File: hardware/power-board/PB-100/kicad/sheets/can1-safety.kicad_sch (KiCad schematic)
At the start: 2 parts

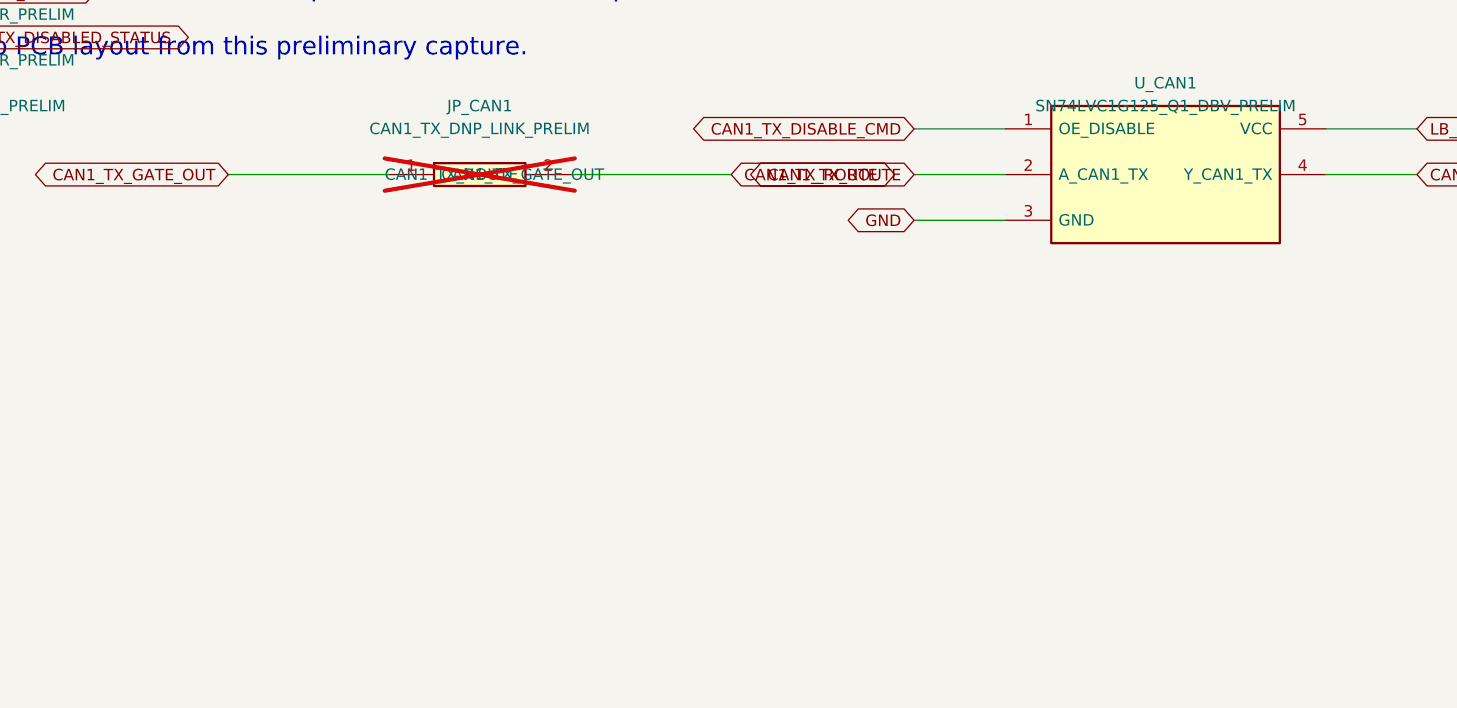
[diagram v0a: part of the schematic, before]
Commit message: fix
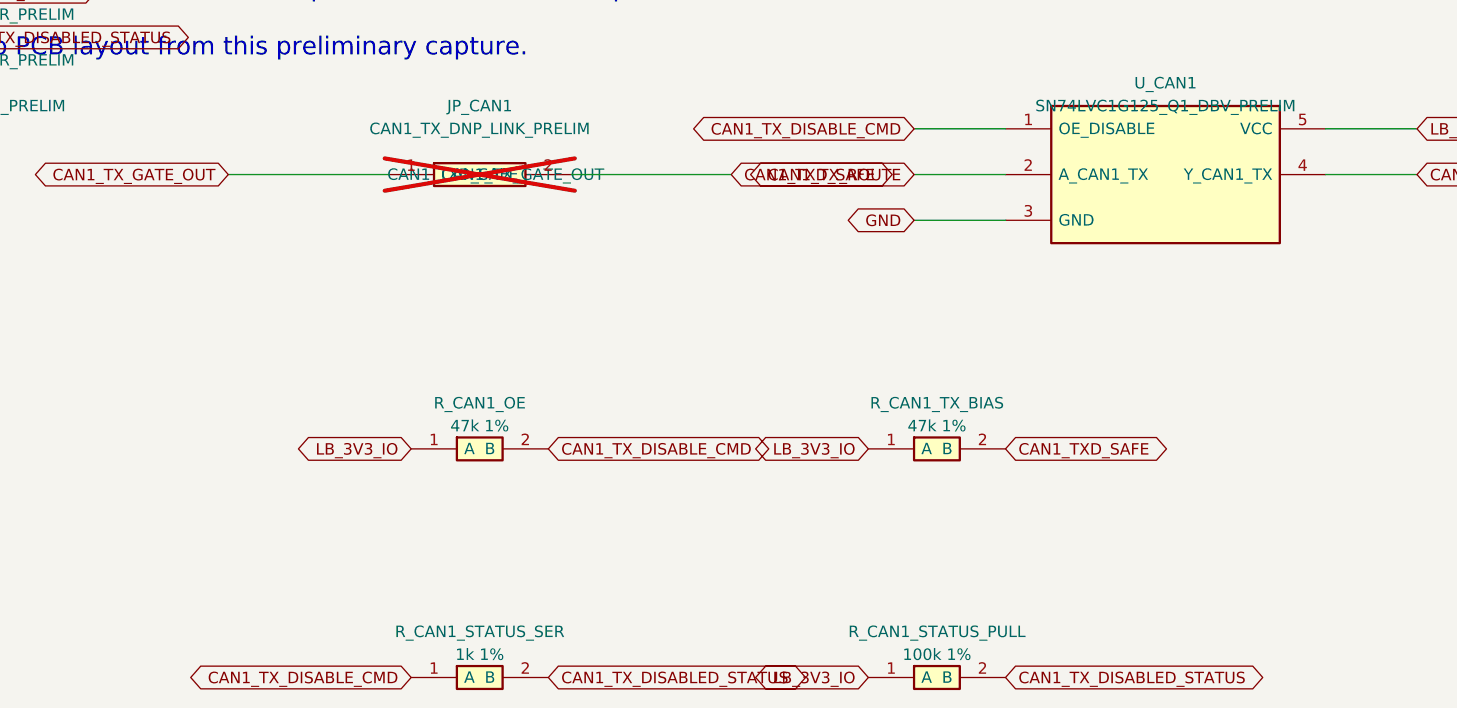
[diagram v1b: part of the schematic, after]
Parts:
- added R_CAN1_OE, R_CAN1_TX_BIAS: 47k 1%, PB100:R0402, symbol PB100:PB100_CAN1_SAFETY_RESISTOR_PRELIM
- added R_CAN1_STATUS_PULL: 100k 1%, PB100:R0402, symbol PB100:PB100_CAN1_SAFETY_RESISTOR_PRELIM
- added R_CAN1_STATUS_SER: 1k 1%, PB100:R0402, symbol PB100:PB100_CAN1_SAFETY_RESISTOR_PRELIM
- JP_CAN1: footprint (none) -> PB100:R0603_DNP_LINK_1608Metric
- U_CAN1: footprint (none) -> PB100:SOT-23-5_DBV_TI
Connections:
- net CAN1_TX_DISABLED_STATUS: now also R_CAN1_STATUS_PULL.2 (B), R_CAN1_STATUS_SER.2 (B)
- net CAN1_TX_DISABLE_CMD: now also R_CAN1_OE.2 (B), R_CAN1_STATUS_SER.1 (A)
- net CAN1_TX_ROUTE: no longer JP_CAN1.2 (CAN1_TX_ROUTE)
- net LB_3V3_IO: now also R_CAN1_OE.1 (A), R_CAN1_STATUS_PULL.1 (A), R_CAN1_TX_BIAS.1 (A)
- new net CAN1_TXD_SAFE: JP_CAN1.2 (CAN1_TXD_SAFE), R_CAN1_TX_BIAS.2 (B)
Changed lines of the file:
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@@
     (property "Reference" "JP_CAN1" (at 76.20 53.34 0) (effects (font (size 1.27 1.27))))
     (property "Value" "CAN1_TX_DNP_LINK_PRELIM" (at 76.20 55.88 0) (effects (font (size 1.27 1.27))))
-    (property "Footprint" "" (at 76.20 66.04 0) (effects (font (size 1.27 1.27)) hide))
+    (property "Footprint" "PB100:R0603_DNP_LINK_1608Metric" (at 76.20 66.04 0) (effects (font (size 1.27 1.27)) hide))
     (property "Datasheet" "../PB-100-can1-tx-disable.md" (at 76.20 68.58 0) (effects (font (size 1.27 1.27)) hide))
     (pin "1")
@@
   (global_label "CAN1_TX_GATE_OUT" (shape bidirectional) (at 48.26 60.96 0) (fields_autoplaced) (effects (font (size 1.27 1.27)) (justify right)) (property "Intersheetrefs" "${INTERSHEET_REFS}" (at 48.26 60.96 0) (effects (font (size 1.27 1.27)) hide)))
   (wire (pts (xy 86.36 60.96) (xy 104.14 60.96)) (stroke (width 0) (type default)))
-  (global_label "CAN1_TX_ROUTE" (shape bidirectional) (at 104.14 60.96 0) (fields_autoplaced) (effects (font (size 1.27 1.27)) (justify left)) (property "Intersheetrefs" "${INTERSHEET_REFS}" (at 104.14 60.96 0) (effects (font (size 1.27 1.27)) hide)))
+  (global_label "CAN1_TXD_SAFE" (shape bidirectional) (at 104.14 60.96 0) (fields_autoplaced) (effects (font (size 1.27 1.27)) (justify left)) (property "Intersheetrefs" "${INTERSHEET_REFS}" (at 104.14 60.96 0) (effects (font (size 1.27 1.27)) hide)))
   (symbol
     (lib_id "PB100:PB100_SN74LVC1G125_Q1_DBV_PRELIM")
@@
     (property "Reference" "U_CAN1" (at 152.40 50.80 0) (effects (font (size 1.27 1.27))))
     (property "Value" "SN74LVC1G125_Q1_DBV_PRELIM" (at 152.40 53.34 0) (effects (font (size 1.27 1.27))))
-    (property "Footprint" "" (at 152.40 71.12 0) (effects (font (size 1.27 1.27)) hide))
+    (property "Footprint" "PB100:SOT-23-5_DBV_TI" (at 152.40 71.12 0) (effects (font (size 1.27 1.27)) hide))
     (property "Datasheet" "https://www.ti.com/lit/ds/symlink/sn74lvc1g125-q1.pdf" (at 152.40 73.66 0) (effects (font (size 1.27 1.27)) hide))
     (pin "1")
@@
   (global_label "LB_3V3_IO" (shape bidirectional) (at 180.34 55.88 0) (fields_autoplaced) (effects (font (size 1.27 1.27)) (justify left)) (property "Intersheetrefs" "${INTERSHEET_REFS}" (at 180.34 55.88 0) (effects (font (size 1.27 1.27)) hide)))
   (symbol
+    (lib_id "PB100:PB100_CAN1_SAFETY_RESISTOR_PRELIM")
+    (at 76.20 91.44 0)
+    (unit 1)
+    (exclude_from_sim no)
+    (in_bom yes)
+    (on_board yes)
+    (dnp no)
+    (property "Reference" "R_CAN1_OE" (at 76.20 86.36 0) (effects (font (size 1.27 1.27))))
+    (property "Value" "47k 1%" (at 76.20 88.90 0) (effects (font (size 1.27 1.27))))
+    (property "Footprint" "PB100:R0402" (at 76.20 96.52 0) (effects (font (size 1.27 1.27)) hide))
+    (property "Datasheet" "../PB-100-can1-tx-disable-design-calculation.md" (at 76.20 99.06 0) (effects (font (size 1.27 1.27)) hide))
+    (pin "1")
+    (pin "2")
+    (instances
+      (project "PB-100"
+        (path "/1af68b81-10b0-5461-9124-39421a2a6932/80055f99-6297-4ce2-96ea-d333e2a69a50/"
+          (reference "R_CAN1_OE")
+          (unit 1)
+        )
+      )
+    )
+  )
+  (global_label "LB_3V3_IO" (shape bidirectional) (at 68.58 91.44 0) (fields_autoplaced) (effects (font (size 1.27 1.27)) (justify right)) (property "Intersheetrefs" "${INTERSHEET_REFS}" (at 68.58 91.44 0) (effects (font (size 1.27 1.27)) hide)))
+  (global_label "CAN1_TX_DISABLE_CMD" (shape bidirectional) (at 83.82 91.44 0) (fields_autoplaced) (effects (font (size 1.27 1.27)) (justify left)) (property "Intersheetrefs" "${INTERSHEET_REFS}" (at 83.82 91.44 0) (effects (font (size 1.27 1.27)) hide)))
+  (symbol
+    (lib_id "PB100:PB100_CAN1_SAFETY_RESISTOR_PRELIM")
+    (at 127.00 91.44 0)
+    (unit 1)
+    (exclude_from_sim no)
+    (in_bom yes)
+    (on_board yes)
+    (dnp no)
+    (property "Reference" "R_CAN1_TX_BIAS" (at 127.00 86.36 0) (effects (font (size 1.27 1.27))))
+    (property "Value" "47k 1%" (at 127.00 88.90 0) (effects (font (size 1.27 1.27))))
+    (property "Footprint" "PB100:R0402" (at 127.00 96.52 0) (effects (font (size 1.27 1.27)) hide))
+    (property "Datasheet" "../PB-100-can1-tx-disable-design-calculation.md" (at 127.00 99.06 0) (effects (font (size 1.27 1.27)) hide))
+    (pin "1")
+    (pin "2")
+    (instances
+      (project "PB-100"
+        (path "/1af68b81-10b0-5461-9124-39421a2a6932/8b75beab-22de-42a1-ba89-68e9bd2ad844/"
+          (reference "R_CAN1_TX_BIAS")
+          (unit 1)
+        )
+      )
+    )
+  )
+  (global_label "LB_3V3_IO" (shape bidirectional) (at 119.38 91.44 0) (fields_autoplaced) (effects (font (size 1.27 1.27)) (justify right)) (property "Intersheetrefs" "${INTERSHEET_REFS}" (at 119.38 91.44 0) (effects (font (size 1.27 1.27)) hide)))
+  (global_label "CAN1_TXD_SAFE" (shape bidirectional) (at 134.62 91.44 0) (fields_autoplaced) (effects (font (size 1.27 1.27)) (justify left)) (property "Intersheetrefs" "${INTERSHEET_REFS}" (at 134.62 91.44 0) (effects (font (size 1.27 1.27)) hide)))
+  (symbol
+    (lib_id "PB100:PB100_CAN1_SAFETY_RESISTOR_PRELIM")
+    (at 76.20 116.84 0)
+    (unit 1)
+    (exclude_from_sim no)
+    (in_bom yes)
+    (on_board yes)
+    (dnp no)
+    (property "Reference" "R_CAN1_STATUS_SER" (at 76.20 111.76 0) (effects (font (size 1.27 1.27))))
+    (property "Value" "1k 1%" (at 76.20 114.30 0) (effects (font (size 1.27 1.27))))
+    (property "Footprint" "PB100:R0402" (at 76.20 121.92 0) (effects (font (size 1.27 1.27)) hide))
+    (property "Datasheet" "../PB-100-can1-tx-disable-design-calculation.md" (at 76.20 124.46 0) (effects (font (size 1.27 1.27)) hide))
+    (pin "1")
+    (pin "2")
+    (instances
+      (project "PB-100"
+        (path "/1af68b81-10b0-5461-9124-39421a2a6932/32b2e633-ddfb-4068-9ee8-5caed1060666/"
+          (reference "R_CAN1_STATUS_SER")
+          (unit 1)
+        )
+      )
+    )
+  )
+  (global_label "CAN1_TX_DISABLE_CMD" (shape bidirectional) (at 68.58 116.84 0) (fields_autoplaced) (effects (font (size 1.27 1.27)) (justify right)) (property "Intersheetrefs" "${INTERSHEET_REFS}" (at 68.58 116.84 0) (effects (font (size 1.27 1.27)) hide)))
+  (global_label "CAN1_TX_DISABLED_STATUS" (shape bidirectional) (at 83.82 116.84 0) (fields_autoplaced) (effects (font (size 1.27 1.27)) (justify left)) (property "Intersheetrefs" "${INTERSHEET_REFS}" (at 83.82 116.84 0) (effects (font (size 1.27 1.27)) hide)))
+  (symbol
+    (lib_id "PB100:PB100_CAN1_SAFETY_RESISTOR_PRELIM")
+    (at 127.00 116.84 0)
+    (unit 1)
+    (exclude_from_sim no)
+    (in_bom yes)
+    (on_board yes)
+    (dnp no)
+    (property "Reference" "R_CAN1_STATUS_PULL" (at 127.00 111.76 0) (effects (font (size 1.27 1.27))))
+    (property "Value" "100k 1%" (at 127.00 114.30 0) (effects (font (size 1.27 1.27))))
+    (property "Footprint" "PB100:R0402" (at 127.00 121.92 0) (effects (font (size 1.27 1.27)) hide))
+    (property "Datasheet" "../PB-100-can1-tx-disable-design-calculation.md" (at 127.00 124.46 0) (effects (font (size 1.27 1.27)) hide))
+    (pin "1")
+    (pin "2")
+    (instances
+      (project "PB-100"
+        (path "/1af68b81-10b0-5461-9124-39421a2a6932/ac9557eb-9bb9-41f8-b23a-db6800c089e1/"
+          (reference "R_CAN1_STATUS_PULL")
+          (unit 1)
+        )
+      )
+    )
+  )
+  (global_label "LB_3V3_IO" (shape bidirectional) (at 119.38 116.84 0) (fields_autoplaced) (effects (font (size 1.27 1.27)) (justify right)) (property "Intersheetrefs" "${INTERSHEET_REFS}" (at 119.38 116.84 0) (effects (font (size 1.27 1.27)) hide)))
+  (global_label "CAN1_TX_DISABLED_STATUS" (shape bidirectional) (at 134.62 116.84 0) (fields_autoplaced) (effects (font (size 1.27 1.27)) (justify left)) (property "Intersheetrefs" "${INTERSHEET_REFS}" (at 134.62 116.84 0) (effects (font (size 1.27 1.27)) hide)))
+  (symbol
     (lib_id "PB100:PB100_ERC_SIGNAL_DRIVER_PRELIM")
